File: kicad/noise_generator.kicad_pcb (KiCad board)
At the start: 2 copper layers, 57.2 x 38.1 mm, 12 parts, among them J1 Conn_Coaxial, J2 Connector, U1 LM741

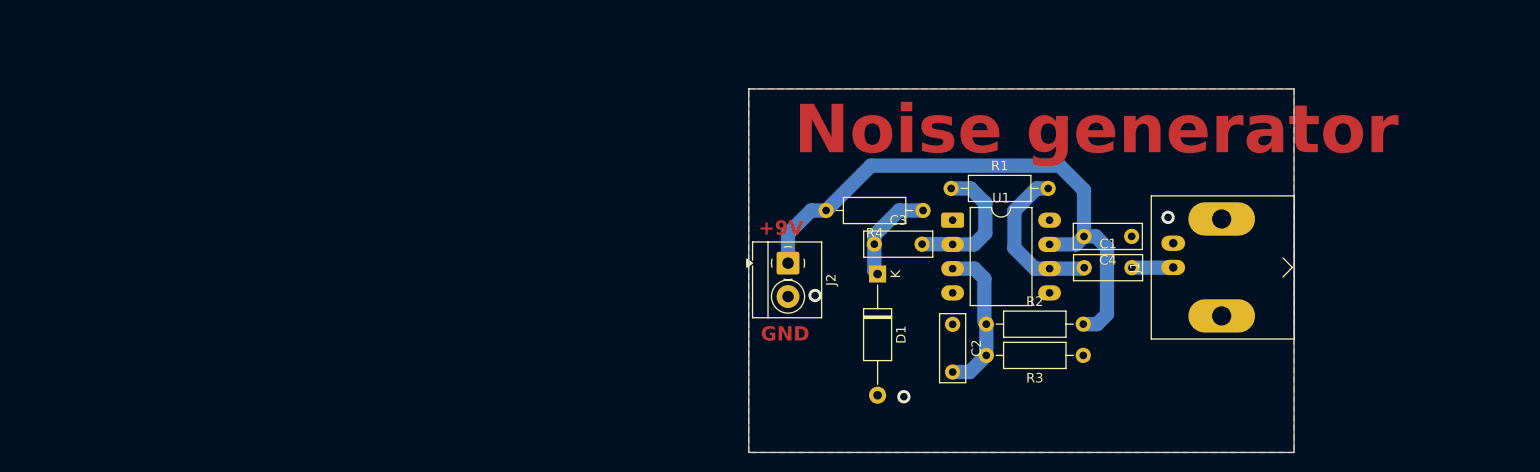
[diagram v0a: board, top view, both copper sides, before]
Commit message: Adjustments
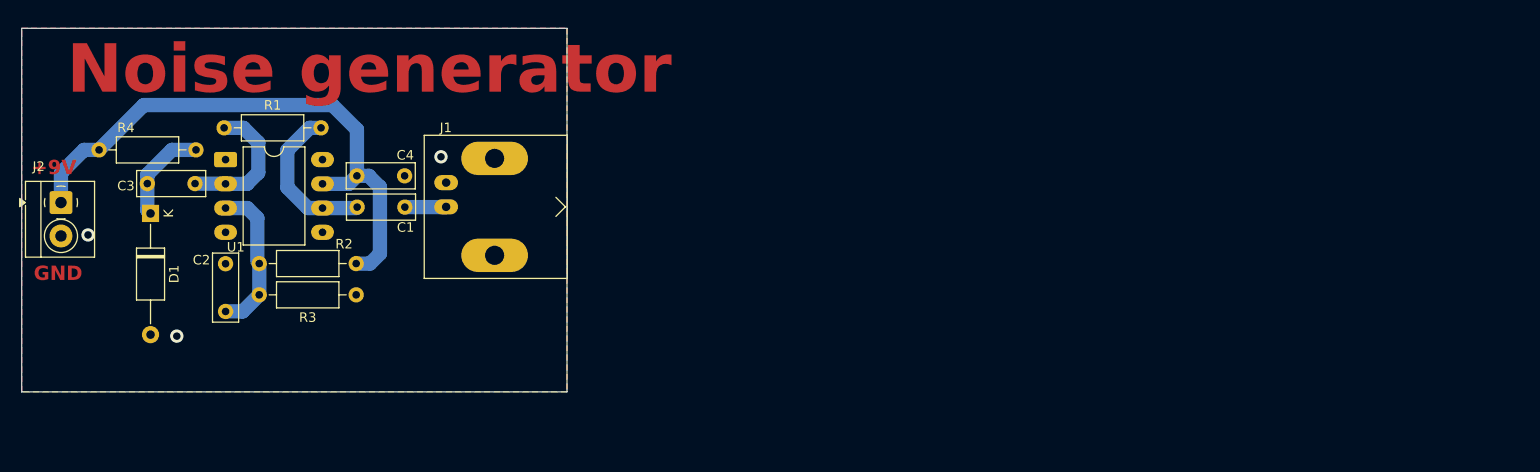
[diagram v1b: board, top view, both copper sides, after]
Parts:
- moved C1 76.5 mm to (130.4, 82.2)
- moved C2 76.5 mm to (116.6, 88.2)
- moved C3 76.5 mm to (108.4, 79.8)
- moved D1 76.5 mm to (108.8, 82.9)
- moved R1 76.5 mm to (116.5, 73.9)
- moved R2 76.5 mm to (120.1, 88.2)
- moved U1 76.5 mm to (116.6, 77.3)
- moved C4 76.5 mm to (135.4, 79.0)
- moved J1 76.5 mm to (139.7, 82.2)
- moved J2 76.5 mm to (99.4, 81.8)
- moved R3 76.5 mm to (130.3, 91.4)
- moved R4 76.5 mm to (113.5, 76.2)
